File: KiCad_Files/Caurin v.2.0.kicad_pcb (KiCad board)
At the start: 4 copper layers, 86 x 86 mm, 73 parts, among them IC1 L7806ABD2T-TR, J1 ESQ-120-39-G-D, J2 Conn_01x12_Male, J3 Conn_01x09_Male, J4 CONSMA001-SMD-G, J5 CONSMA001-SMD-G, J6 U_FL-R-SMT_10_, J7 CONSMA001-SMD-G, J8 MEM2075-00-140-01-A, J9 Conn_01x02_Male, Q1 PMT280ENEAX, U1 STM32L476RGTx, U2 2AD66-1262, U3 LoRa1262F30, U5 NEO-M8N, U6 W25Q32JVSSIQ_TR, U7 TCAN330G, Y1 32,768k

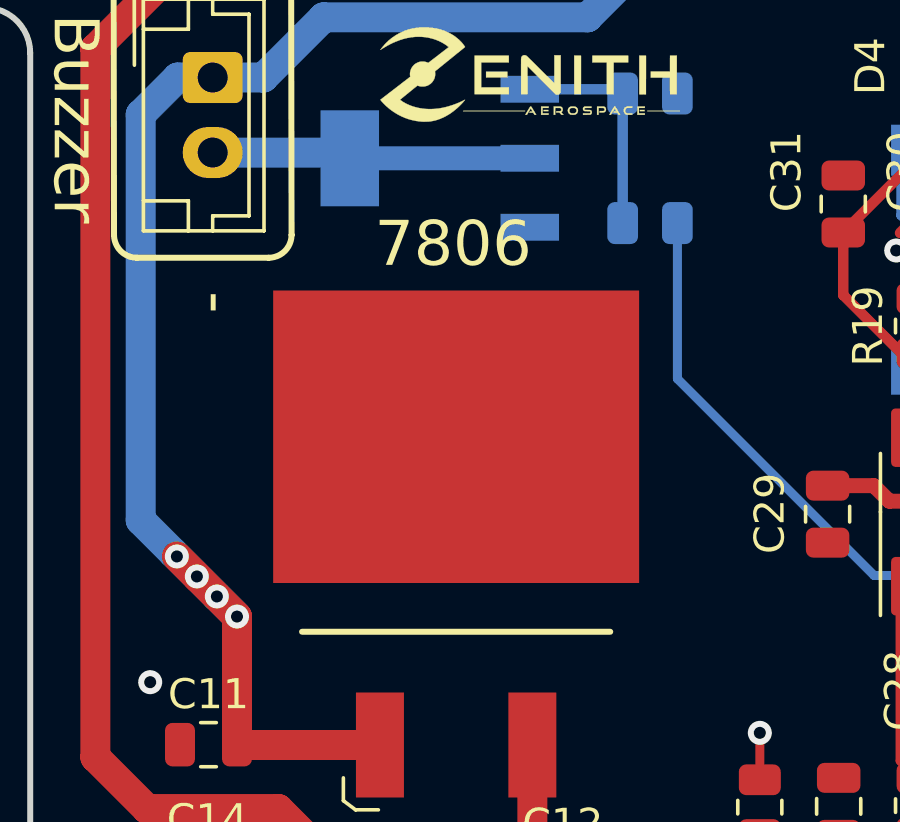
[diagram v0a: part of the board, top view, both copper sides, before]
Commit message: Update 7806 Traces
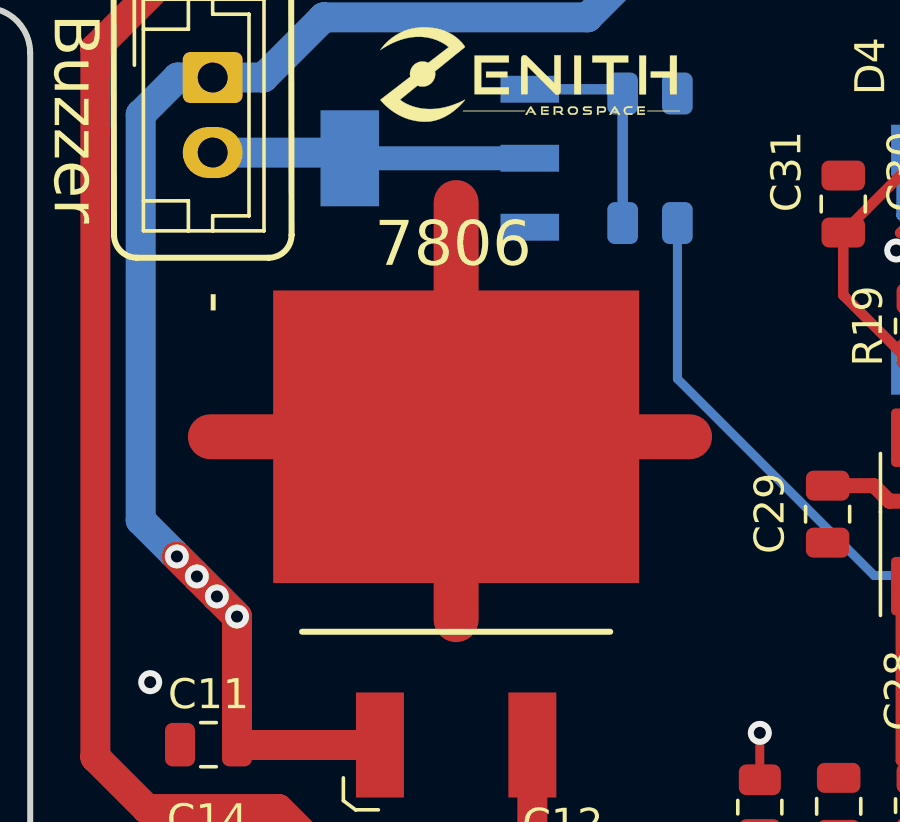
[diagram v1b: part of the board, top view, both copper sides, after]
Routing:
- net GND: track 90.3 -> 120.2 mm
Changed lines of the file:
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@@
     (thickness 1.6)
     (drawings 422)
-    (tracks 1233)
+    (tracks 1237)
     (zones 0)
     (modules 73)
@@
   )
   (setup
-    (last_trace_width 0.5)
+    (last_trace_width 1.5)
     (user_trace_width 0.2)
     (user_trace_width 0.25)
@@
     (add_net UART_TX)
   )
+  (module Crystal:Crystal_SMD_3215-2Pin_3.2x1.5mm (layer F.Cu)
+    (at 165.5064 77.89672 180)
+    (descr "SMD Crystal FC-135 https://support.epson.biz/td/api/doc_check.php?dl=brief_FC-135R_en.pdf")
+    (tags "SMD SMT Crystal")
+    (attr smd)
+    (fp_text reference Y1 (at 0 -2.11328) (layer F.SilkS) hide
+      (effects (font (size 1 1) (thickness 0.15)))
+    )
+    (fp_text value 32,768k (at 0 2) (layer F.Fab)
+      (effects (font (size 1 1) (thickness 0.15)))
+    )
+    (fp_line (start 2 -1.15) (end 2 1.15) (layer F.CrtYd) (width 0.05))
+    (fp_line (start -2 -1.15) (end -2 1.15) (layer F.CrtYd) (width 0.05))
+    (fp_line (start -2 1.15) (end 2 1.15) (layer F.CrtYd) (width 0.05))
+    (fp_line (start -1.6 0.75) (end 1.6 0.75) (layer F.Fab) (width 0.1))
+    (fp_line (start -1.6 -0.75) (end 1.6 -0.75) (layer F.Fab) (width 0.1))
+    (fp_line (start 1.6 -0.75) (end 1.6 0.75) (layer F.Fab) (width 0.1))
+    (fp_line (start -0.675 -0.875) (end 0.675 -0.875) (layer F.SilkS) (width 0.12))
+    (fp_line (start -0.675 0.875) (end 0.675 0.875) (layer F.SilkS) (width 0.12))
+    (fp_line (start -1.6 -0.75) (end -1.6 0.75) (layer F.Fab) (width 0.1))
+    (fp_line (start -2 -1.15) (end 2 -1.15) (layer F.CrtYd) (width 0.05))
+    (fp_text user %R (at 0 -2) (layer F.Fab)
+      (effects (font (size 1 1) (thickness 0.15)))
+    )
+    (pad 2 smd rect (at -1.25 0 180) (size 1 1.8) (layers F.Cu F.Paste F.Mask)
+      (net 6 LSE_IN))
+    (pad 1 smd rect (at 1.25 0 180) (size 1 1.8) (layers F.Cu F.Paste F.Mask)
+      (net 7 LSE_OUT))
+    (model ${KISYS3DMOD}/Crystal.3dshapes/Crystal_SMD_MicroCrystal_CC7V-T1A-2Pin_3.2x1.5mm.step
+      (at (xyz 0 0 0))
+      (scale (xyz 1 1 1))
+      (rotate (xyz 0 0 0))
+    )
+  )
   (module RF_Modules_Zenith:2AD66-126x (layer B.Cu)
     (at 143.2664 119.7356 270)
@@
       (effects (font (size 1 1) (thickness 0.15)))
     )
-    (fp_text user %R (at 0 0 180) (layer F.Fab)
-      (effects (font (size 1 1) (thickness 0.15)))
-    )
     (fp_line (start -2.3 -1.6) (end 2.3 -1.6) (layer F.Fab) (width 0.1))
     (fp_line (start 2.3 -1.6) (end 2.5 -1.4) (layer F.Fab) (width 0.1))
@@
     (fp_line (start 2.8 1.9) (end 2.8 -1.9) (layer F.CrtYd) (width 0.05))
     (fp_line (start 2.8 -1.9) (end -2.8 -1.9) (layer F.CrtYd) (width 0.05))
+    (fp_text user %R (at 0 0 180) (layer F.Fab)
+      (effects (font (size 1 1) (thickness 0.15)))
+    )
     (pad 4 smd roundrect (at -1.65 -1 180) (size 2 1.5) (layers F.Cu F.Paste F.Mask) (roundrect_rratio 0.1)
       (net 1 GND))
@@
     )
   )
-  (module Crystal:Crystal_SMD_3215-2Pin_3.2x1.5mm (layer F.Cu)
-    (at 165.5064 77.89672 180)
-    (descr "SMD Crystal FC-135 https://support.epson.biz/td/api/doc_check.php?dl=brief_FC-135R_en.pdf")
-    (tags "SMD SMT Crystal")
-    (attr smd)
-    (fp_text reference Y1 (at 0 -2.11328 180) (layer F.SilkS) hide
-      (effects (font (size 1 1) (thickness 0.15)))
-    )
-    (fp_text value 32,768k (at 0 2 180) (layer F.Fab)
-      (effects (font (size 1 1) (thickness 0.15)))
-    )
-    (fp_line (start 2 -1.15) (end 2 1.15) (layer F.CrtYd) (width 0.05))
-    (fp_line (start -2 -1.15) (end -2 1.15) (layer F.CrtYd) (width 0.05))
-    (fp_line (start -2 1.15) (end 2 1.15) (layer F.CrtYd) (width 0.05))
-    (fp_line (start -1.6 0.75) (end 1.6 0.75) (layer F.Fab) (width 0.1))
-    (fp_line (start -1.6 -0.75) (end 1.6 -0.75) (layer F.Fab) (width 0.1))
-    (fp_line (start 1.6 -0.75) (end 1.6 0.75) (layer F.Fab) (width 0.1))
-    (fp_line (start -0.675 -0.875) (end 0.675 -0.875) (layer F.SilkS) (width 0.12))
-    (fp_line (start -0.675 0.875) (end 0.675 0.875) (layer F.SilkS) (width 0.12))
-    (fp_line (start -1.6 -0.75) (end -1.6 0.75) (layer F.Fab) (width 0.1))
-    (fp_line (start -2 -1.15) (end 2 -1.15) (layer F.CrtYd) (width 0.05))
-    (fp_text user %R (at 0 -2 180) (layer F.Fab)
-      (effects (font (size 1 1) (thickness 0.15)))
-    )
-    (pad 2 smd rect (at -1.25 0 180) (size 1 1.8) (layers F.Cu F.Paste F.Mask)
-      (net 6 LSE_IN))
-    (pad 1 smd rect (at 1.25 0 180) (size 1 1.8) (layers F.Cu F.Paste F.Mask)
-      (net 7 LSE_OUT))
-    (model ${KISYS3DMOD}/Crystal.3dshapes/Crystal_SMD_3215-2Pin_3.2x1.5mm.wrl
-      (at (xyz 0 0 0))
-      (scale (xyz 1 1 1))
-      (rotate (xyz 0 0 0))
-    )
-    (model ${KISYS3DMOD}/Crystal.3dshapes/Crystal_SMD_MicroCrystal_CC7V-T1A-2Pin_3.2x1.5mm.step
-      (at (xyz 0 0 0))
-      (scale (xyz 1 1 1))
-      (rotate (xyz 0 0 0))
-    )
-  )
   (module SamacSys_Parts:YC164JR07220RL (layer B.Cu)
     (at 179.2605 96.0755)
@@
   (via (at 127.3175 120.396) (size 0.8) (drill 0.4) (layers F.Cu B.Cu) (net 1))
   (via (at 128.2065 121.3485) (size 0.8) (drill 0.4) (layers F.Cu B.Cu) (net 1))
+  (segment (start 124.4981 84.9738) (end 124.4981 77.1652) (width 1.5) (layer F.Cu) (net 1))
+  (segment (start 124.4981 84.9738) (end 132.2813 84.9738) (width 1.5) (layer F.Cu) (net 1))
+  (segment (start 124.4981 84.9738) (end 116.3047 84.9738) (width 1.5) (layer F.Cu) (net 1))
+  (segment (start 124.4981 84.9738) (end 124.4981 91.0717) (width 1.5) (layer F.Cu) (net 1))
   (segment (start 154.8384 76.05542) (end 155.2204 75.67342) (width 0.3) (layer F.Cu) (net 2))
   (segment (start 154.8384 77.89672) (end 154.8384 76.05542) (width 0.3) (layer F.Cu) (net 2))
